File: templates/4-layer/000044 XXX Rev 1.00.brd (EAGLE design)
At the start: 259 x 228 mm, 22 parts, among them X1 PAD_TEST_GROUND_HOOK

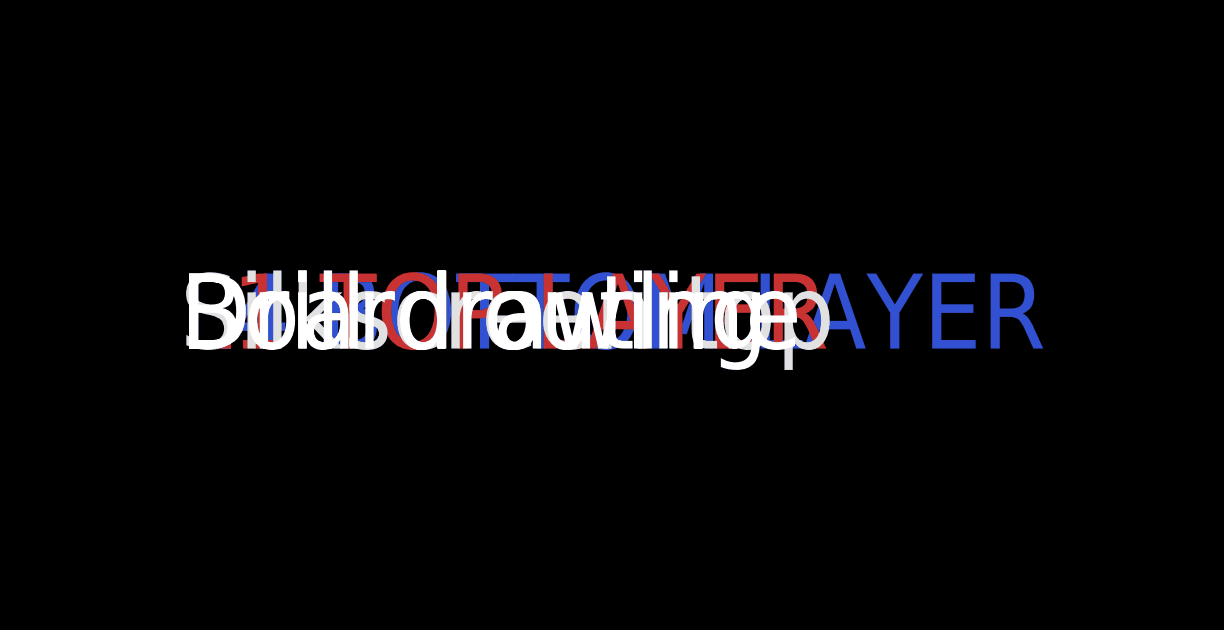
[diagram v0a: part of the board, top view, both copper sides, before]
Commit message: bugfixes
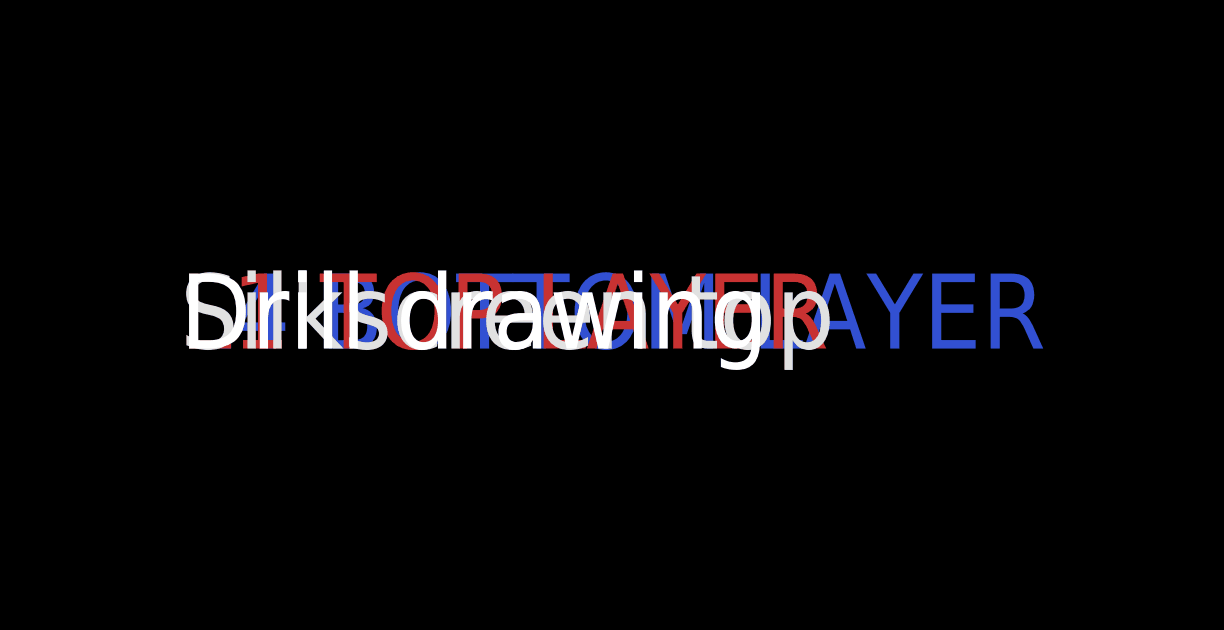
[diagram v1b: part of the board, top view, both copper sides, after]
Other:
- board text removed: "Board outline"
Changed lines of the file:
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@@
 <text x="133" y="27" size="2.5" layer="1" font="vector" ratio="12" align="top-left">L1 TOP LAYER</text>
 <text x="133" y="27" size="2.5" layer="2" font="vector" ratio="12" align="top-left">L2 mid-layer</text>
-<text x="133" y="27" size="2.5" layer="20" font="vector" ratio="12" align="top-left">Board outline</text>
 <text x="-21.5" y="6" size="1" layer="2" font="vector" ratio="15" align="center">2</text>
 <text x="-20.5" y="6" size="1" layer="15" font="vector" ratio="15" align="center">3</text>
